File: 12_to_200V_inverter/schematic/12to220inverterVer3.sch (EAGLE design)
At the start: 243 parts, among them IC1 UC3842, IC10 TL494, IC2 PC817, IC3 LM358SOIC8, IC4 TL431, IC5 LM317, IC6 74HC595, IC7 74HC595, IC8 ATTINY45, IC9 TL431, J1 0, J2 0, T1 AO4407AL, T10 16N60, T11 BC847, T12 BC847, T13 BSS84, T15 BC847, T16 BSS84, T17 BC847, T18 BC847, T19 BSS84, T2 IRF830, T20 BSS84, T21 BC847, T22 BC847, T23 BSS84, T24 BC847, T3 IRF830, T4 BC847, T5 BC857, T6 BC857, T7 IRFZ24N, T8 IRFZ24N, T9 BC857, X1 BAT+, X2 LAMP1, X3 LAMP1, X4 BAT-, X5 220VAC, X6 LAMP1_SWITCH, X7 LAMP1_SWITCH, X8 MCU_PROGRAMMING

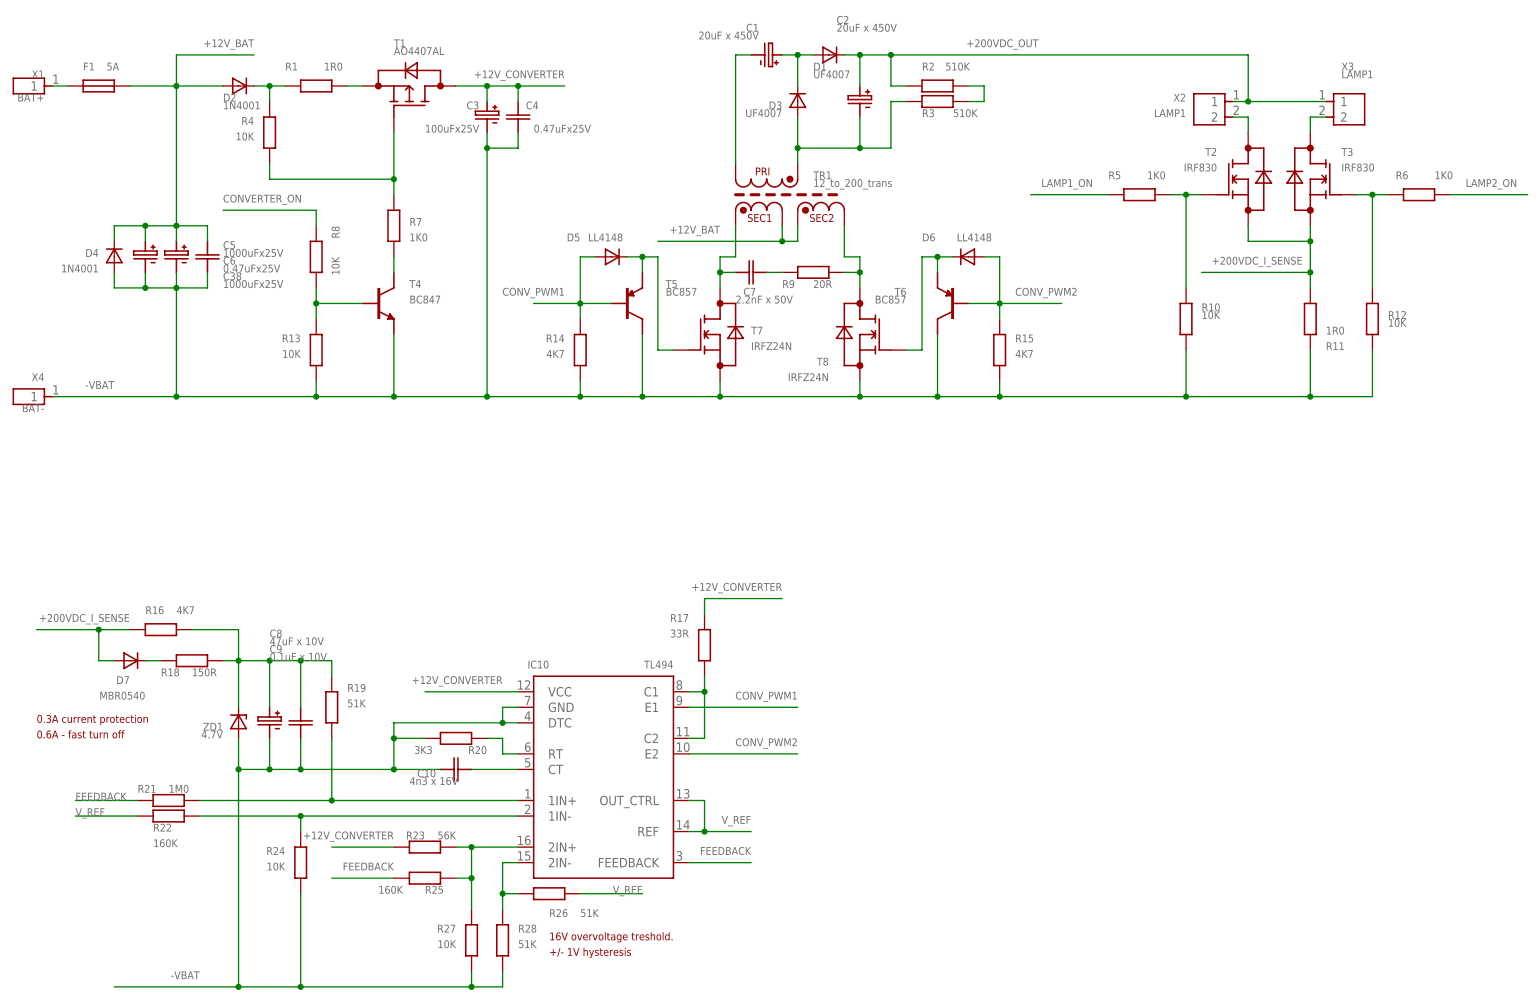
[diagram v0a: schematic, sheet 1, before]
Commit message: 12 to 200V converter. Ver3. Routing.
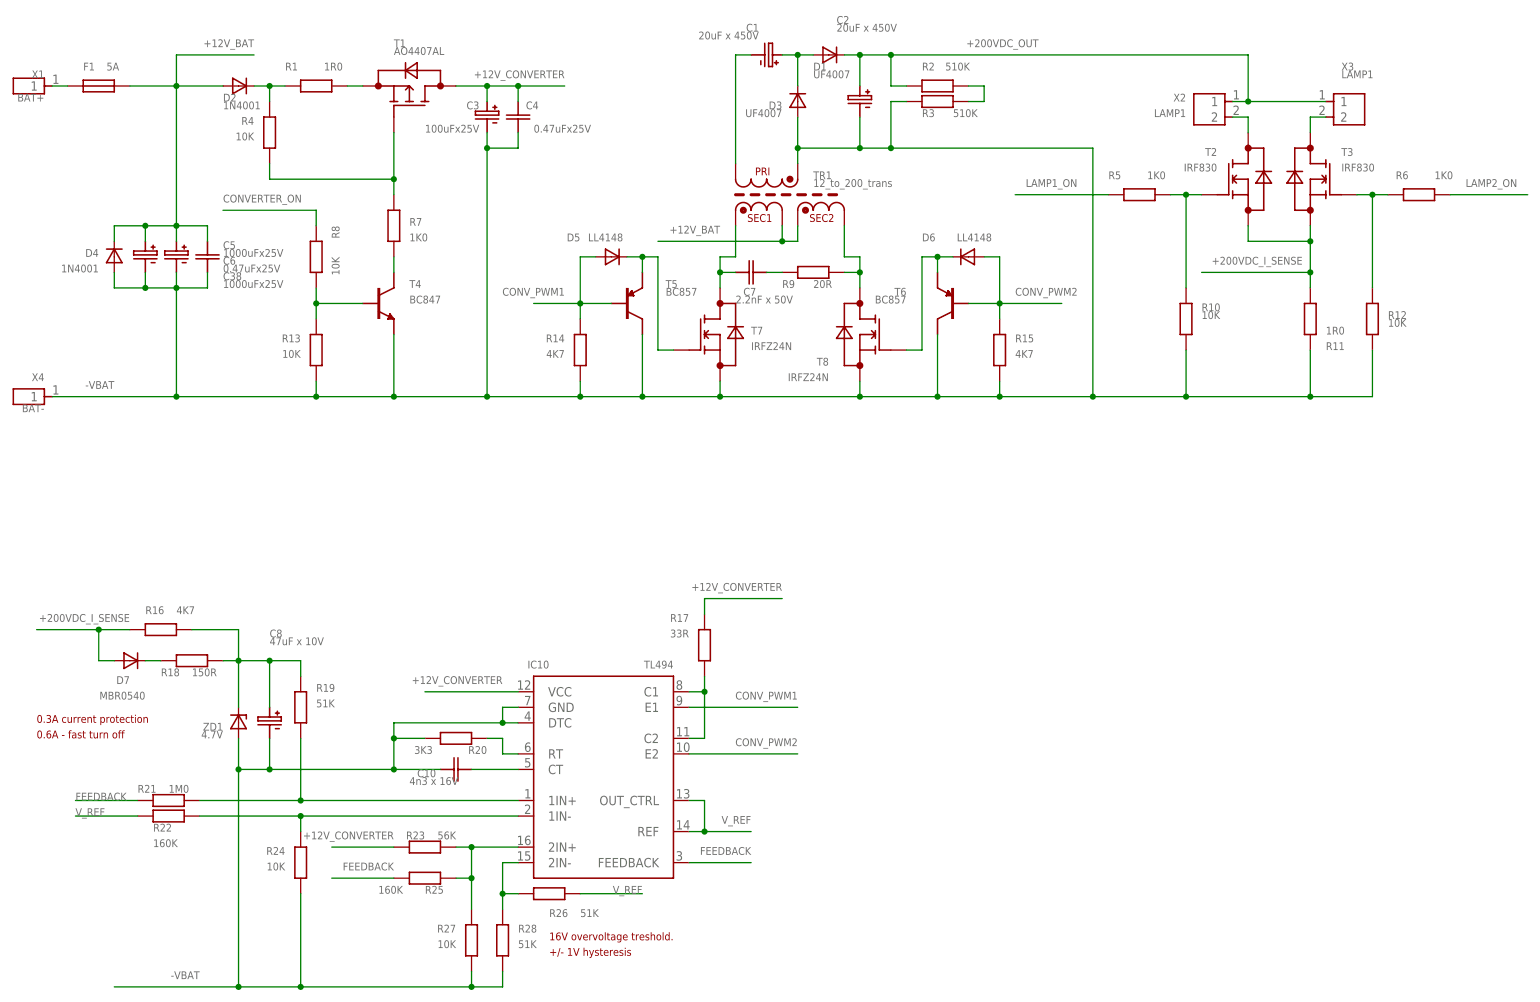
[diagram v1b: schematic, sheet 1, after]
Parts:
- removed C9: 0.1uF x 10V, __MyCommonLib1:CSMD_0805
- D1, D3: device __MyCommonLib1:1N4001DO-41_10MM -> __MyCommonLib1:1N4001DO-41_5MM
- R11: device __MyCommonLib1:R1.0W_VERT -> __MyCommonLib1:R1.0W
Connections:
- removed net N$15: C2.MINUS, D3.ANODE, R3.PIN0, TR1.PRI_START
- net -VBAT: now also C2.MINUS, D3.ANODE, R3.PIN0, TR1.PRI_START; no longer C9.PIN1
- net N$7: no longer C9.PIN0
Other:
- moved on the sheet: R19
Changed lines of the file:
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@@
 <part name="R9" library="__MyCommonLib1" deviceset="R" device="SMD_1206" value="20R"/>
 <part name="C1" library="__MyCommonLib1" deviceset="CE" device="13MM" value="20uF x 450V"/>
-<part name="D3" library="__MyCommonLib1" deviceset="1N4001" device="DO-41_10MM" value="UF4007"/>
-<part name="R11" library="__MyCommonLib1" deviceset="R" device="1.0W_VERT" value="1R0"/>
+<part name="D3" library="__MyCommonLib1" deviceset="1N4001" device="DO-41_5MM" value="UF4007"/>
+<part name="R11" library="__MyCommonLib1" deviceset="R" device="1.0W" value="1R0"/>
 <part name="C4" library="__MyCommonLib1" deviceset="C" device="SMD_0805" value="0.47uFx25V"/>
 <part name="C3" library="__MyCommonLib1" deviceset="CE" device="6.3MM" value="100uFx25V"/>
@@
 <part name="R26" library="__MyCommonLib1" deviceset="R" device="SMD_0805" value="51K"/>
 <part name="ZD1" library="__MyCommonLib1" deviceset="ZENNER" device="(SOD_80)" value="4.7V"/>
-<part name="D1" library="__MyCommonLib1" deviceset="1N4001" device="DO-41_10MM" value="UF4007"/>
+<part name="D1" library="__MyCommonLib1" deviceset="1N4001" device="DO-41_5MM" value="UF4007"/>
 <part name="C2" library="__MyCommonLib1" deviceset="CE" device="13MM" value="20uF x 450V"/>
 <part name="R27" library="__MyCommonLib1" deviceset="R" device="SMD_0805" value="10K"/>
@@
 <part name="D7" library="__MyCommonLib1" deviceset="LL4147" device="SOD-80" value="MBR0540"/>
 <part name="R18" library="__MyCommonLib1" deviceset="R" device="SMD_0805" value="150R"/>
-<part name="C9" library="__MyCommonLib1" deviceset="C" device="SMD_0805" value="0.1uF x 10V"/>
 <part name="FRAME1" library="frames" deviceset="A4L-LOC" device="" value="12_TO_200VDC_CONVERTER"/>
 <part name="X5" library="__MyCommonLib1" deviceset="PIN1X2" device="BRD_CONN_12X10.2" value="220VAC"/>
@@
 <attribute name="VALUE" x="31.75" y="46.99" size="1.27" layer="96" font="vector" ratio="20"/>
 </instance>
-<instance part="R19" gate="R$1" x="58.42" y="60.96" smashed="yes" rot="R180">
-<attribute name="NAME" x="60.96" y="63.5" size="1.27" layer="95" font="vector" ratio="20"/>
-<attribute name="VALUE" x="60.96" y="60.96" size="1.27" layer="96" font="vector" ratio="20"/>
+<instance part="R19" gate="R$1" x="53.34" y="60.96" smashed="yes" rot="R180">
+<attribute name="NAME" x="55.88" y="63.5" size="1.27" layer="95" font="vector" ratio="20"/>
+<attribute name="VALUE" x="55.88" y="60.96" size="1.27" layer="96" font="vector" ratio="20"/>
 </instance>
 <instance part="D7" gate="D1" x="25.4" y="68.58" smashed="yes" rot="R270">
@@
 <attribute name="NAME" x="30.48" y="66.04" size="1.27" layer="95" font="vector" ratio="20"/>
 <attribute name="VALUE" x="35.56" y="66.04" size="1.27" layer="96" font="vector" ratio="20"/>
-</instance>
-<instance part="C9" gate="C$1" x="53.34" y="58.42" smashed="yes" rot="MR180">
-<attribute name="NAME" x="48.26" y="71.12" size="1.27" layer="95" font="vector" ratio="20" rot="MR180"/>
-<attribute name="VALUE" x="48.26" y="69.85" size="1.27" layer="96" font="vector" ratio="20" rot="MR180"/>
 </instance>
 <instance part="T2" gate="G$1" x="205.74" y="147.32" smashed="yes">
@@
 <pinref part="D4" gate="D$1" pin="CATHODE"/>
 <wire x1="22.86" y1="137.16" x2="22.86" y2="139.7" width="0.1524" layer="91"/>
+<pinref part="C6" gate="C$1" pin="PIN1"/>
 <wire x1="22.86" y1="139.7" x2="27.94" y2="139.7" width="0.1524" layer="91"/>
-<pinref part="C6" gate="C$1" pin="PIN1"/>
 <wire x1="27.94" y1="139.7" x2="33.02" y2="139.7" width="0.1524" layer="91"/>
 <wire x1="33.02" y1="139.7" x2="38.1" y2="139.7" width="0.1524" layer="91"/>
 <wire x1="38.1" y1="139.7" x2="38.1" y2="137.16" width="0.1524" layer="91"/>
+<junction x="33.02" y="139.7"/>
 <pinref part="C38" gate="C$1" pin="PLUS"/>
-<wire x1="27.94" y1="139.7" x2="27.94" y2="137.16" width="0.1524" layer="91"/>
-<junction x="33.02" y="139.7"/>
+<wire x1="27.94" y1="137.16" x2="27.94" y2="139.7" width="0.1524" layer="91"/>
 <junction x="27.94" y="139.7"/>
 </segment>
@@
 <net name="N$7" class="0">
 <segment>
-<wire x1="58.42" y1="68.58" x2="53.34" y2="68.58" width="0.1524" layer="91"/>
 <wire x1="53.34" y1="68.58" x2="48.26" y2="68.58" width="0.1524" layer="91"/>
 <wire x1="48.26" y1="68.58" x2="48.26" y2="60.96" width="0.1524" layer="91"/>
@@
 <pinref part="C8" gate="C$1" pin="PLUS"/>
 <pinref part="R19" gate="R$1" pin="PIN0"/>
-<wire x1="58.42" y1="66.04" x2="58.42" y2="68.58" width="0.1524" layer="91"/>
+<wire x1="53.34" y1="66.04" x2="53.34" y2="68.58" width="0.1524" layer="91"/>
 <pinref part="R18" gate="R$1" pin="PIN0"/>
 <wire x1="40.64" y1="68.58" x2="43.18" y2="68.58" width="0.1524" layer="91"/>
-<pinref part="C9" gate="C$1" pin="PIN0"/>
-<wire x1="53.34" y1="60.96" x2="53.34" y2="68.58" width="0.1524" layer="91"/>
-<junction x="53.34" y="68.58"/>
 </segment>
 </net>
@@
 <segment>
 <pinref part="IC10" gate="G$1" pin="1IN+"/>
-<wire x1="88.9" y1="45.72" x2="58.42" y2="45.72" width="0.1524" layer="91"/>
+<wire x1="88.9" y1="45.72" x2="53.34" y2="45.72" width="0.1524" layer="91"/>
 <pinref part="R21" gate="R$1" pin="PIN0"/>
 <pinref part="R19" gate="R$1" pin="PIN1"/>
-<wire x1="58.42" y1="45.72" x2="36.83" y2="45.72" width="0.1524" layer="91"/>
-<wire x1="58.42" y1="55.88" x2="58.42" y2="45.72" width="0.1524" layer="91"/>
-<junction x="58.42" y="45.72"/>
+<wire x1="53.34" y1="45.72" x2="36.83" y2="45.72" width="0.1524" layer="91"/>
+<wire x1="53.34" y1="55.88" x2="53.34" y2="45.72" width="0.1524" layer="91"/>
+<junction x="53.34" y="45.72"/>
 </segment>
 </net>
@@
 <pinref part="ZD1" gate="G$1" pin="ANODE"/>
 <wire x1="43.18" y1="50.8" x2="43.18" y2="55.88" width="0.1524" layer="91"/>
-<pinref part="C9" gate="C$1" pin="PIN1"/>
-<wire x1="53.34" y1="50.8" x2="53.34" y2="55.88" width="0.1524" layer="91"/>
 <wire x1="43.18" y1="50.8" x2="48.26" y2="50.8" width="0.1524" layer="91"/>
-<wire x1="48.26" y1="50.8" x2="53.34" y2="50.8" width="0.1524" layer="91"/>
 <wire x1="48.26" y1="50.8" x2="48.26" y2="55.88" width="0.1524" layer="91"/>
 <pinref part="C8" gate="C$1" pin="MINUS"/>
@@
 <wire x1="68.58" y1="55.88" x2="68.58" y2="50.8" width="0.1524" layer="91"/>
 <wire x1="68.58" y1="50.8" x2="76.2" y2="50.8" width="0.1524" layer="91"/>
-<wire x1="53.34" y1="50.8" x2="68.58" y2="50.8" width="0.1524" layer="91"/>
-<junction x="53.34" y="50.8"/>
+<wire x1="48.26" y1="50.8" x2="68.58" y2="50.8" width="0.1524" layer="91"/>
 <junction x="68.58" y="50.8"/>
 <pinref part="R20" gate="R$1" pin="PIN0"/>
@@
 <junction x="83.82" y="111.76"/>
 <pinref part="R11" gate="R$1" pin="PIN1"/>
-<wire x1="167.64" y1="111.76" x2="198.12" y2="111.76" width="0.1524" layer="91"/>
+<wire x1="167.64" y1="111.76" x2="182.88" y2="111.76" width="0.1524" layer="91"/>
+<wire x1="182.88" y1="111.76" x2="198.12" y2="111.76" width="0.1524" layer="91"/>
 <wire x1="198.12" y1="111.76" x2="218.44" y2="111.76" width="0.1524" layer="91"/>
 <wire x1="218.44" y1="111.76" x2="218.44" y2="119.38" width="0.1524" layer="91"/>
@@
 <wire x1="27.94" y1="129.54" x2="22.86" y2="129.54" width="0.1524" layer="91"/>
 <wire x1="22.86" y1="129.54" x2="22.86" y2="132.08" width="0.1524" layer="91"/>
-<pinref part="C38" gate="C$1" pin="MINUS"/>
-<wire x1="27.94" y1="132.08" x2="27.94" y2="129.54" width="0.1524" layer="91"/>
 <pinref part="C6" gate="C$1" pin="PIN0"/>
 <wire x1="38.1" y1="132.08" x2="38.1" y2="129.54" width="0.1524" layer="91"/>
 <wire x1="38.1" y1="129.54" x2="33.02" y2="129.54" width="0.1524" layer="91"/>
+<junction x="33.02" y="129.54"/>
+<pinref part="C38" gate="C$1" pin="MINUS"/>
+<wire x1="27.94" y1="132.08" x2="27.94" y2="129.54" width="0.1524" layer="91"/>
 <junction x="27.94" y="129.54"/>
-<junction x="33.02" y="129.54"/>
-</segment>
-</net>
-<net name="N$15" class="0">
-<segment>
 <pinref part="D3" gate="D$1" pin="ANODE"/>
 <wire x1="134.62" y1="157.48" x2="134.62" y2="152.4" width="0.1524" layer="91"/>
@@
 <junction x="144.78" y="152.4"/>
 <pinref part="TR1" gate="G$1" pin="PRI_START"/>
+<wire x1="149.86" y1="152.4" x2="182.88" y2="152.4" width="0.1524" layer="91"/>
+<wire x1="182.88" y1="152.4" x2="182.88" y2="111.76" width="0.1524" layer="91"/>
+<junction x="182.88" y="111.76"/>
+<junction x="149.86" y="152.4"/>
 </segment>
 </net>
@@
 <segment>
 <pinref part="R5" gate="R$1" pin="PIN1"/>
-<wire x1="185.42" y1="144.78" x2="172.72" y2="144.78" width="0.1524" layer="91"/>
-<label x="182.88" y="147.32" size="1.27" layer="95" font="vector" ratio="20" rot="R180"/>
-</segment>
-</net>
+<wire x1="185.42" y1="144.78" x2="170.18" y2="144.78" width="0.1524" layer="91"/>
+<label x="180.34" y="147.32" size="1.27" layer="95" font="vector" ratio="20" rot="R180"/>
+</segment>
+</net>
